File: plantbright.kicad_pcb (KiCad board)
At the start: 2 copper layers, 34.5 x 48 mm, 21 parts, among them J1 POWER OUT, J2 5V IN, Q1 AO3400A, Q2 AO3400A, Q3 AO3400A, Q5 AO3400A, SW1 USER 0, U1 XIAO-ESP32-C6

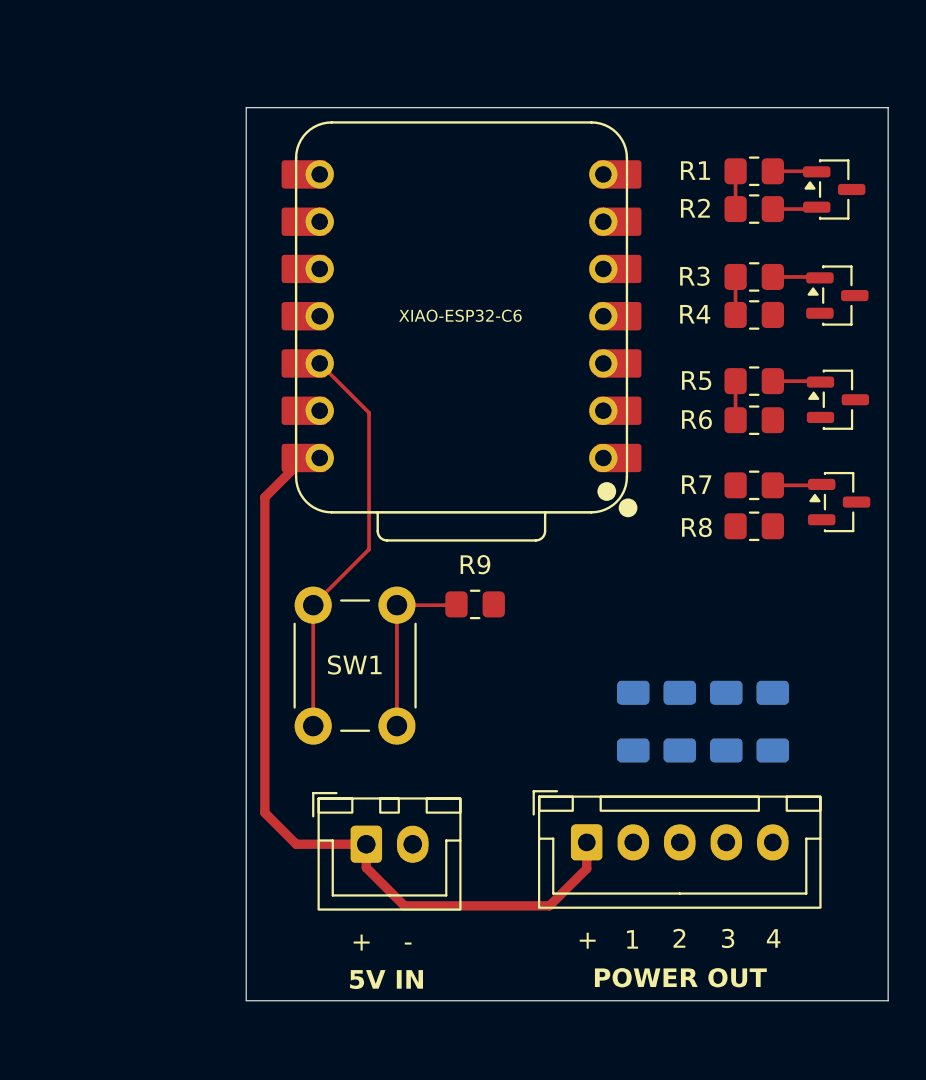
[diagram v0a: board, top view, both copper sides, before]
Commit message: Enough for tonight, I think the shape works.
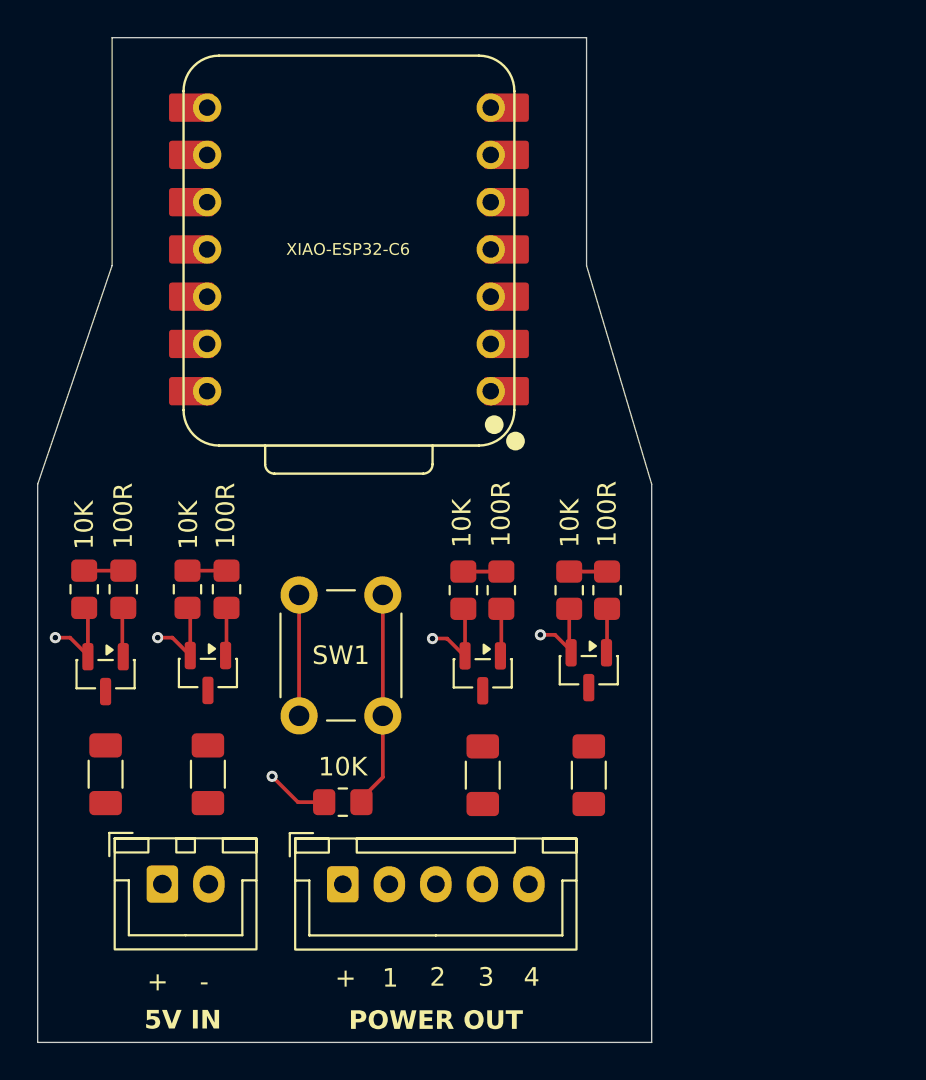
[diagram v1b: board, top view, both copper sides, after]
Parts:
- R10, R11, R12, R13: moved to F.Cu
- moved Q5 40.5 mm to (140.4, 98.5), turned to -90 degrees
- moved Q3 36.9 mm to (145.9, 98.5), turned to -90 degrees
- moved R8 36.2 mm to (139.3, 94.0), turned to -90 degrees
- moved R13 36.0 mm to (140.4, 103.9)
- moved R7 34.4 mm to (141.4, 94.0), turned to -90 degrees
- moved R6 31.8 mm to (144.8, 94.0), turned to -90 degrees
- moved R5 30.5 mm to (146.9, 94.0), turned to -90 degrees
- moved Q1 29.0 mm to (166.4, 98.3), turned to -90 degrees
- moved R12 28.0 mm to (145.9, 103.9)
- moved Q2 27.8 mm to (160.7, 98.5), turned to -90 degrees
- moved R1 23.9 mm to (167.4, 94.0), turned to -90 degrees
- moved R2 22.8 mm to (165.4, 94.0), turned to -90 degrees
- moved R3 21.6 mm to (161.7, 94.0), turned to -90 degrees
- moved R4 21.5 mm to (159.7, 94.0), turned to -90 degrees
- moved J1 13.3 mm to (153.2, 109.8)
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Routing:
- net +5V: track 42.3 -> 0.00 mm
- net GND: track 2.26 -> 22.2 mm, vias 0 -> 5
- net +3.3V: track 21.8 -> 6.50 mm
- net CH_4: track 0.00 -> 2.20 mm
- net BTN_1: track 9.50 -> 11.6 mm
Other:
- board size 34.5 x 48 mm -> 33 x 54 mm
